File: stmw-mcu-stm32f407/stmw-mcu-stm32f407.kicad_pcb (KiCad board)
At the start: 2 copper layers, 70 x 43.5 mm, 41 parts, among them J2 TYPE-C-31-M-12, SW1 TS-1088R-02526, SW2 TS-1088R-02526, U1 AMS1117-3.3, U3 STM32F407VETx, Y1 X_16MHZ

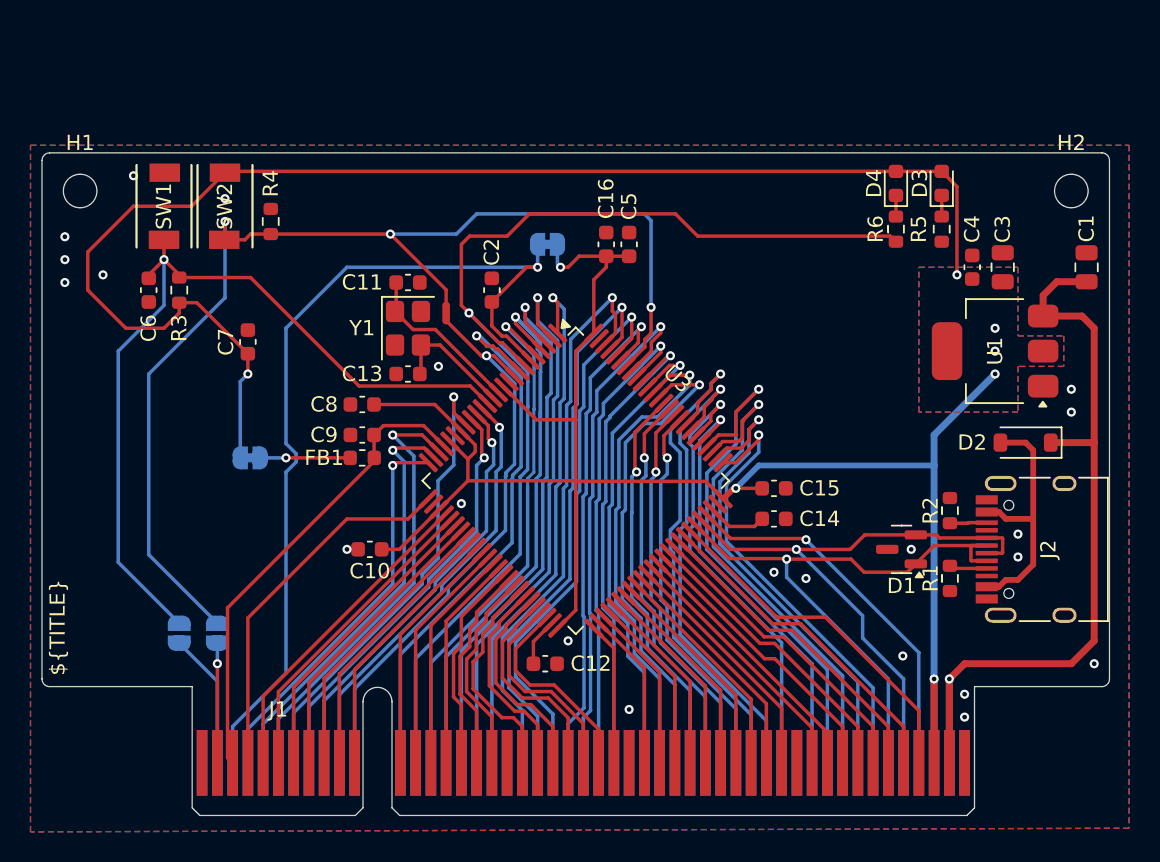
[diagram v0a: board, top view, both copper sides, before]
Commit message: Hmmm
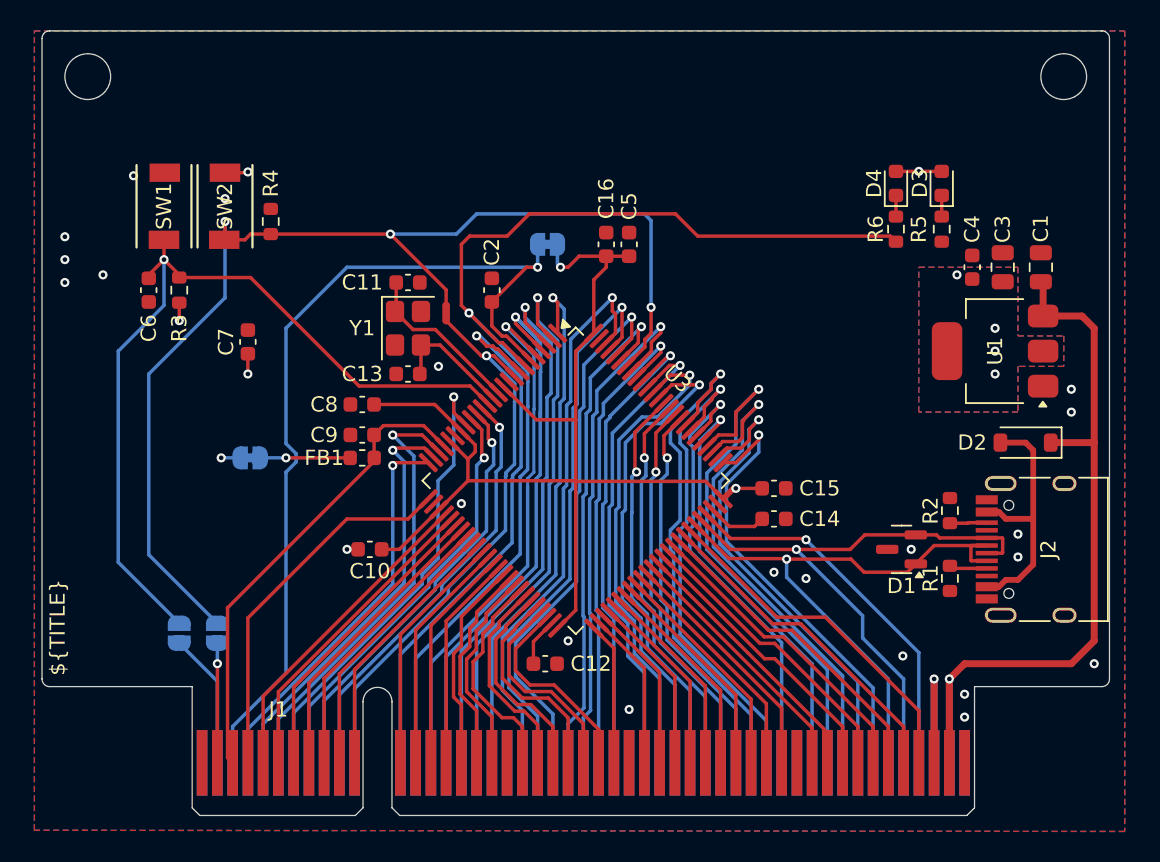
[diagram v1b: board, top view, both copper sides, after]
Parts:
- removed H1, H2: MountingHole, MountingHole:MountingHole_2.2mm_M2
- D3: value LED_GREEN_0603 -> GR
- D4: value LED_BLUE_0603 -> BL
- moved C1 3.00 mm to (180.5, 85.0)
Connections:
- J1 pad A19: U4 -> U1
- J1 pad A27: U6 -> U3
- J1 pad A38: U8 -> U5
- J1 pad B19: U5 -> U2
- J1 pad B27: U7 -> U4
- J1 pad B38: U9 -> U6
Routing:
- net +3V3: track 212.4 -> 96.5 mm, vias 8 -> 12
- net +5V: track 53.1 -> 50.9 mm
- net GND: vias 21 -> 22
- net (no net): vias 1 -> 0
- added copper zone on In1.Cu, net +3V3
- added copper zone on In2.Cu, net GND
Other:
- board size 70 x 43.5 mm -> 70 x 51.5 mm
- copper layers 2 -> 4
